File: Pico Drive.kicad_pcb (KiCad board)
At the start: 2 copper layers, 100.3 x 102.2 mm, 31 parts, among them J1 Conn_01x06_Male, J2 Conn_01x08, J3 Conn_01x02_Male, J4 Conn_01x02_Male, SW1 Reset, U1 Pico, U2 74AXP1T45GWH, U3 74AHCT1G125, U4 OLED-I2C-Module-Aliexpress

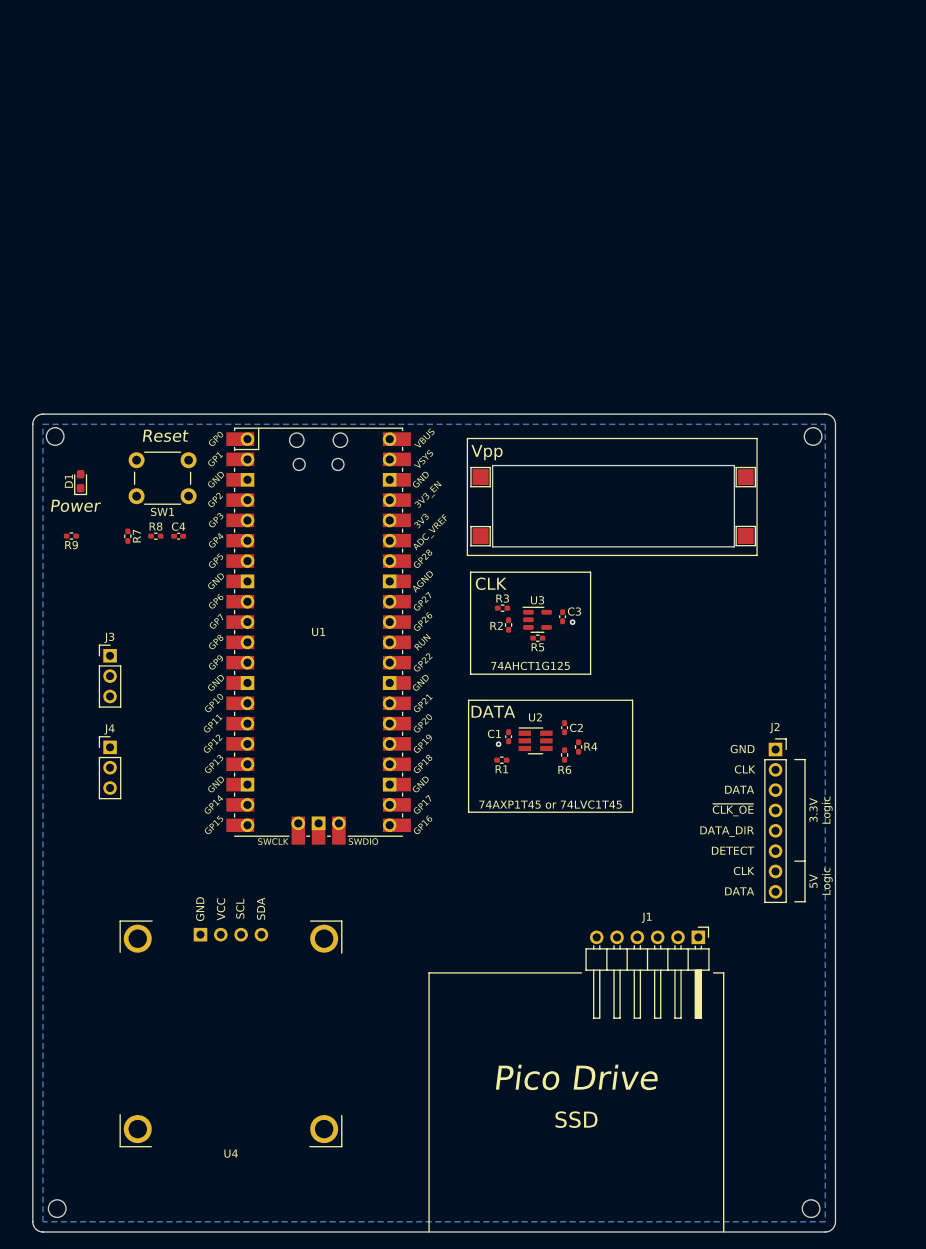
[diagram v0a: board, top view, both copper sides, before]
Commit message: Rotated and shrank the board, tidied stuff up
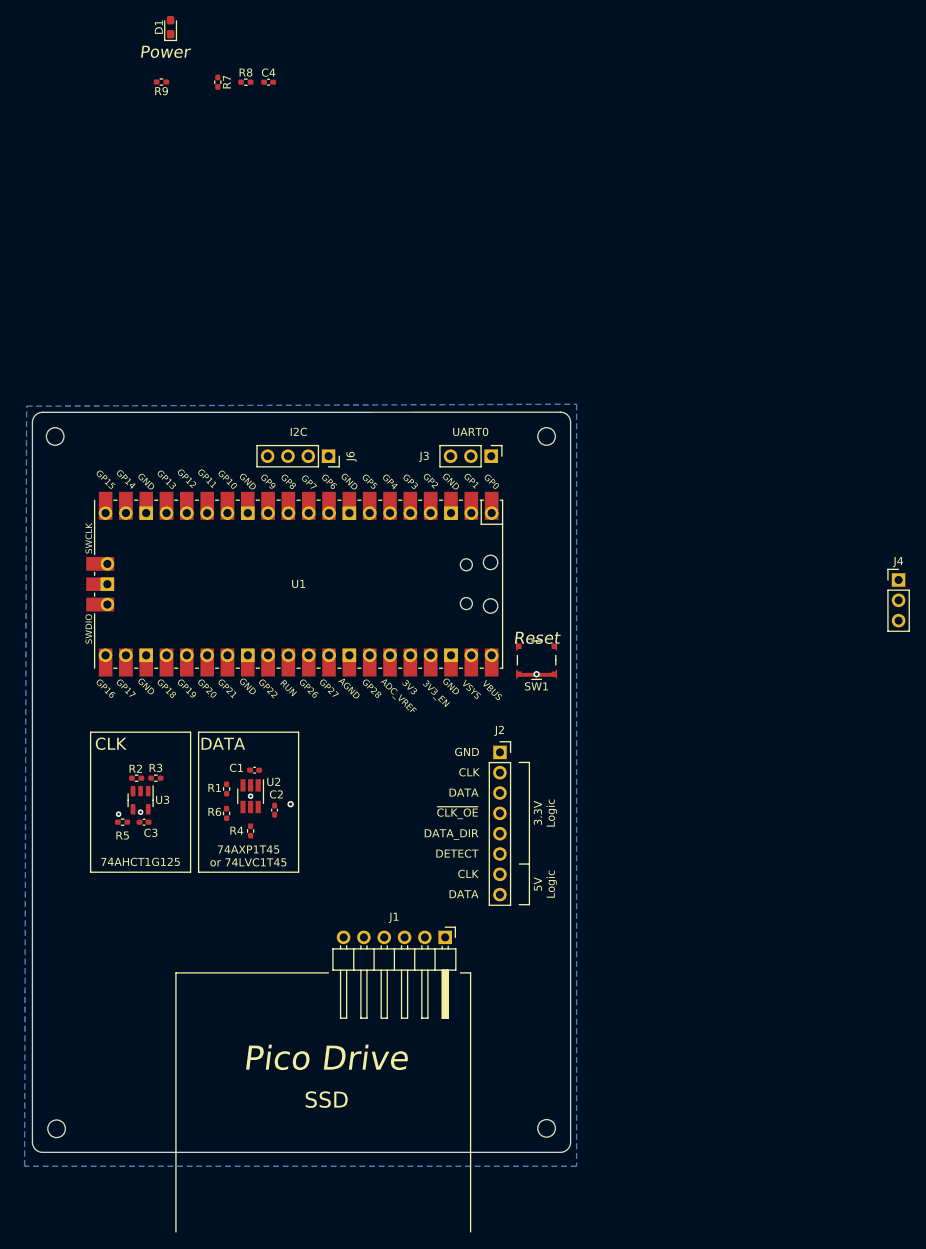
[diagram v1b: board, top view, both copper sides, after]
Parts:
- removed REF** (x4): TestPoint_Pad_2.0x2.0mm, TestPoint:TestPoint_Pad_2.0x2.0mm
- removed U4: OLED-I2C-Module-Aliexpress, kiwih_kicad:OLED-I2C-Module-Aliexpress
- added J6: I2C, Connector_PinSocket_2.54mm:PinSocket_1x04_P2.54mm_Vertical, F.Cu at (54.8, 20.5)
- SW1: footprint Button_Switch_THT:SW_PUSH_6mm -> digikey-footprints:Switch_Tactile_SMD_4.5x4.5mm_TL3315NF160Q
- moved J4 100.8 mm to (126.0, 36.0)
- moved C3 58.3 mm to (31.7, 66.2), turned to 180 degrees
- moved C4 57.9 mm to (47.2, -26.2)
- moved D1 57.9 mm to (35.0, -33.1)
- moved R7 57.9 mm to (40.9, -26.2)
- moved R8 57.9 mm to (44.4, -26.2)
- moved R9 57.9 mm to (33.9, -26.3)
- moved R5 56.8 mm to (29.0, 66.2)
- moved U3 54.5 mm to (31.2, 63.5), turned to -90 degrees
- moved J3 53.8 mm to (75.1, 20.5), turned to -90 degrees
- moved R2 50.3 mm to (30.8, 60.8), turned to 180 degrees
- moved R3 48.3 mm to (33.2, 60.8), turned to 180 degrees
- moved SW1 48.1 mm to (80.8, 46.0)
- moved R6 42.9 mm to (42.0, 65.2)
- moved R4 42.3 mm to (45.0, 67.3)
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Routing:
- net GND: track 0.00 -> 4.00 mm, vias 2 -> 5
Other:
- board size 100.3 x 102.2 mm -> 67.3 x 92.5 mm
- board text added: "I2C"
- board text added: "UART0"
- board text removed: "Vpp"

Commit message: Complete revamp, with routing.
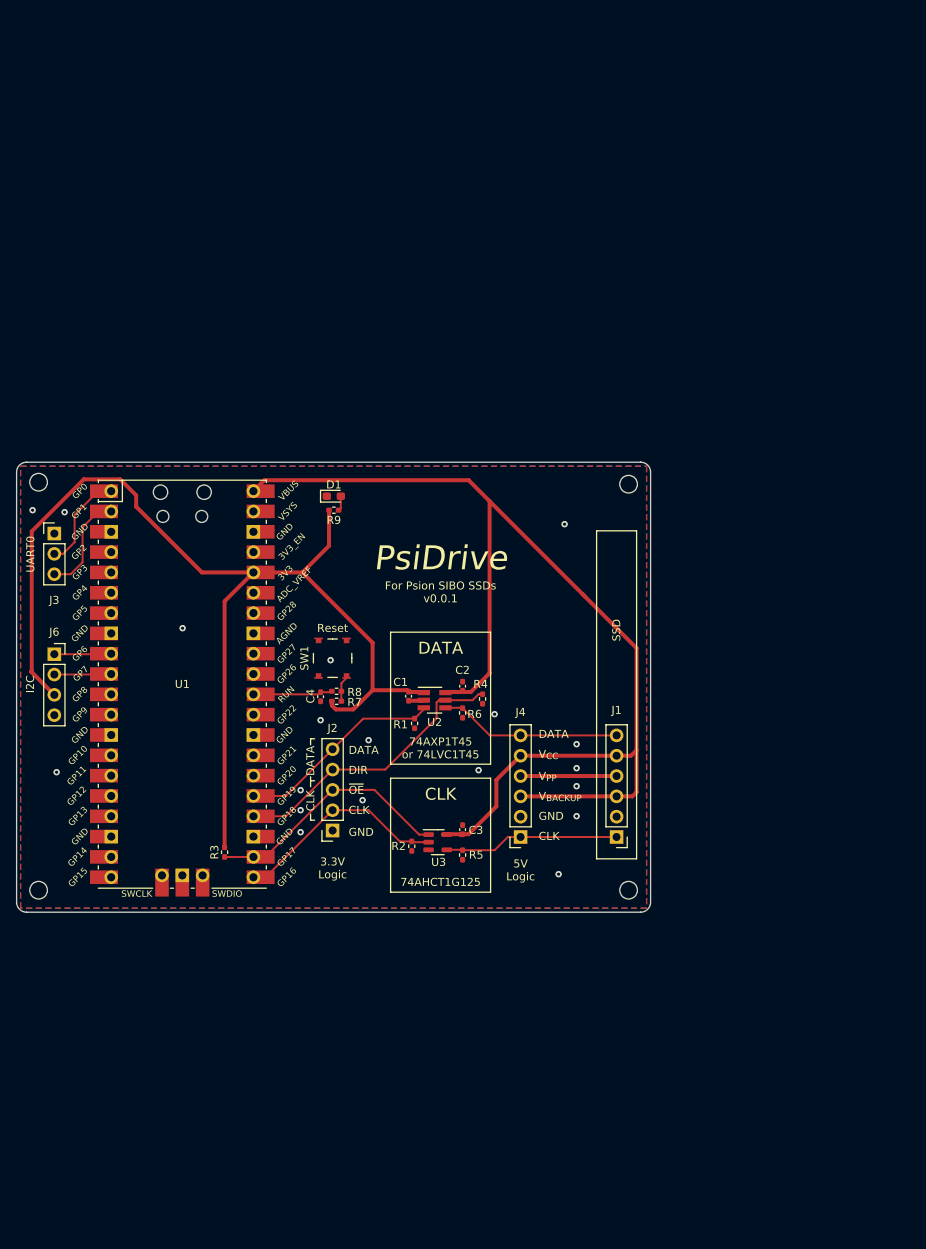
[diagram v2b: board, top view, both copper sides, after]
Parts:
- J1: footprint Connector_PinHeader_2.54mm:PinHeader_1x06_P2.54mm_Horizontal -> Connector_PinHeader_2.54mm:PinHeader_1x06_P2.54mm_Vertical
- J2: value Conn_01x08 -> Conn_01x05; footprint Connector_PinSocket_2.54mm:PinSocket_1x08_P2.54mm_Vertical -> Connector_PinSocket_2.54mm:PinSocket_1x05_P2.54mm_Vertical
- J3: value Conn_01x02_Male -> Conn_01x03_Male
- J4: value Conn_01x02_Male -> Conn_01x06; footprint Connector_PinHeader_2.54mm:PinHeader_1x03_P2.54mm_Vertical -> Connector_PinSocket_2.54mm:PinSocket_1x06_P2.54mm_Vertical
- U3: value 74AHCT1G125 -> 74AHCT1G125DBVTG4
- moved H4 81.2 mm to (92.2, 24.0), turned to 90 degrees
- moved R7 78.8 mm to (55.8, 51.1), turned to 0 degrees
- moved H3 77.5 mm to (92.2, 74.8), turned to 90 degrees
- moved C4 77.1 mm to (53.8, 50.6), turned to -90 degrees
- moved R8 77.0 mm to (55.8, 49.9), turned to 180 degrees
- moved H1 63.8 mm to (18.5, 23.8), turned to 90 degrees
- moved D1 62.1 mm to (55.4, 25.5), turned to 0 degrees
- moved R9 57.7 mm to (55.4, 27.2), turned to 0 degrees
- moved J4 57.1 mm to (78.8, 68.1), turned to 180 degrees
- moved H2 56.8 mm to (18.5, 74.8), turned to 90 degrees
- moved J3 55.5 mm to (20.5, 30.2), turned to 0 degrees
- moved R5 42.7 mm to (71.5, 70.3), turned to -90 degrees
- moved J6 42.3 mm to (20.5, 45.2), turned to 0 degrees
- moved C3 39.8 mm to (71.5, 67.2), turned to 90 degrees
- moved U3 37.5 mm to (68.4, 68.8), turned to 0 degrees
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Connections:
- J1 pad 3: unconnected-(J1-Pad3) -> +5V
- J1 pad 4: unconnected-(J1-Pad4) -> /VDD
- J2 pad 3: /DATA_3V3 -> /~{CLK_OE}
- J2 pad 5: /~{CLK_OE} -> /DATA_3V3
- J4 pad 1: GND -> /CLK_5V
- J4 pad 2: /UART1_TX -> GND
- J4 pad 3: /UART1_RX -> +5V
- U1 pad 22: /DATA_3V3 -> /~{CLK_OE}
- U1 pad 25: /~{CLK_OE} -> /DATA_3V3
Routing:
- net +5V: track 0.05 -> 148.9 mm
- net +3V3: track 0.00 -> 140.5 mm
- net /DATA_DIR: track 0.00 -> 36.1 mm
- net /~{CLK_OE}: track 0.00 -> 31.0 mm
- net /CLK_3V3: track 0.00 -> 26.4 mm
- net /DATA_3V3: track 0.00 -> 26.0 mm
- net /DATA_5V: track 0.00 -> 22.8 mm
- net /CLK_5V: track 0.00 -> 21.9 mm
- net /UART0_RX: track 0.00 -> 12.9 mm
- net /UART0_TX: track 0.00 -> 12.4 mm
- net /VDD: track 0.00 -> 12.0 mm
- net /~{RUN}: track 0.00 -> 9.96 mm
- net /I2C1_SDA: track 0.00 -> 7.13 mm
- net /I2C1_SCL: track 0.00 -> 7.13 mm
- net Net-(R7-Pad2): track 0.00 -> 3.18 mm
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- added copper zone on F.Cu, net GND
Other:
- board size 67.3 x 92.5 mm -> 79.2 x 56.2 mm
- board text added: "DIR"
- board text added: "For Psion SIBO SSDs v0.0.1"
- board text added: "PsiDrive"
- board text added: "V_{BACKUP}"
- board text added: "V_{CC}"
- board text added: "V_{PP}"
- board text added: "~{OE}"
- board text removed: "DATA_DIR"
- board text removed: "DETECT"
- board text removed: "Pico Drive"
- board text removed: "Power"
- board text removed: "~{CLK_OE}"
